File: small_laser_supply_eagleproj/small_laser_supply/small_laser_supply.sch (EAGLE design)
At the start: 25 parts, among them U1 LT6003_SOT23-5, X1 VIN, X2 CTRL, X3 OUT

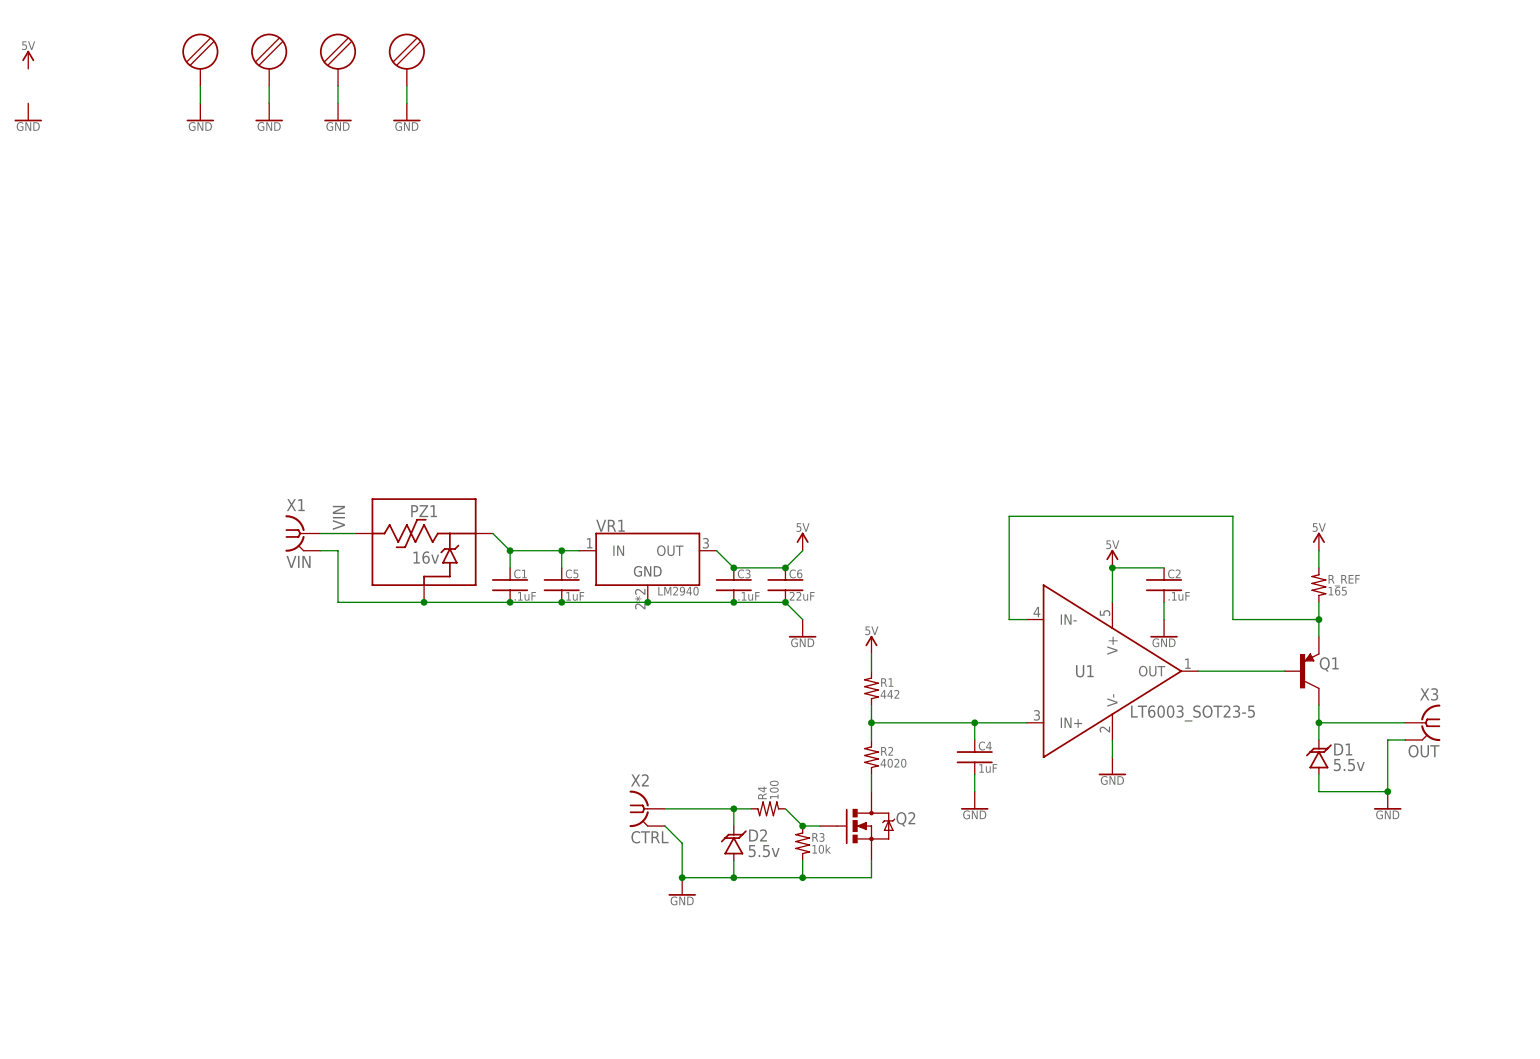
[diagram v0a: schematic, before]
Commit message: Fixed version of the schematic seems to be finished
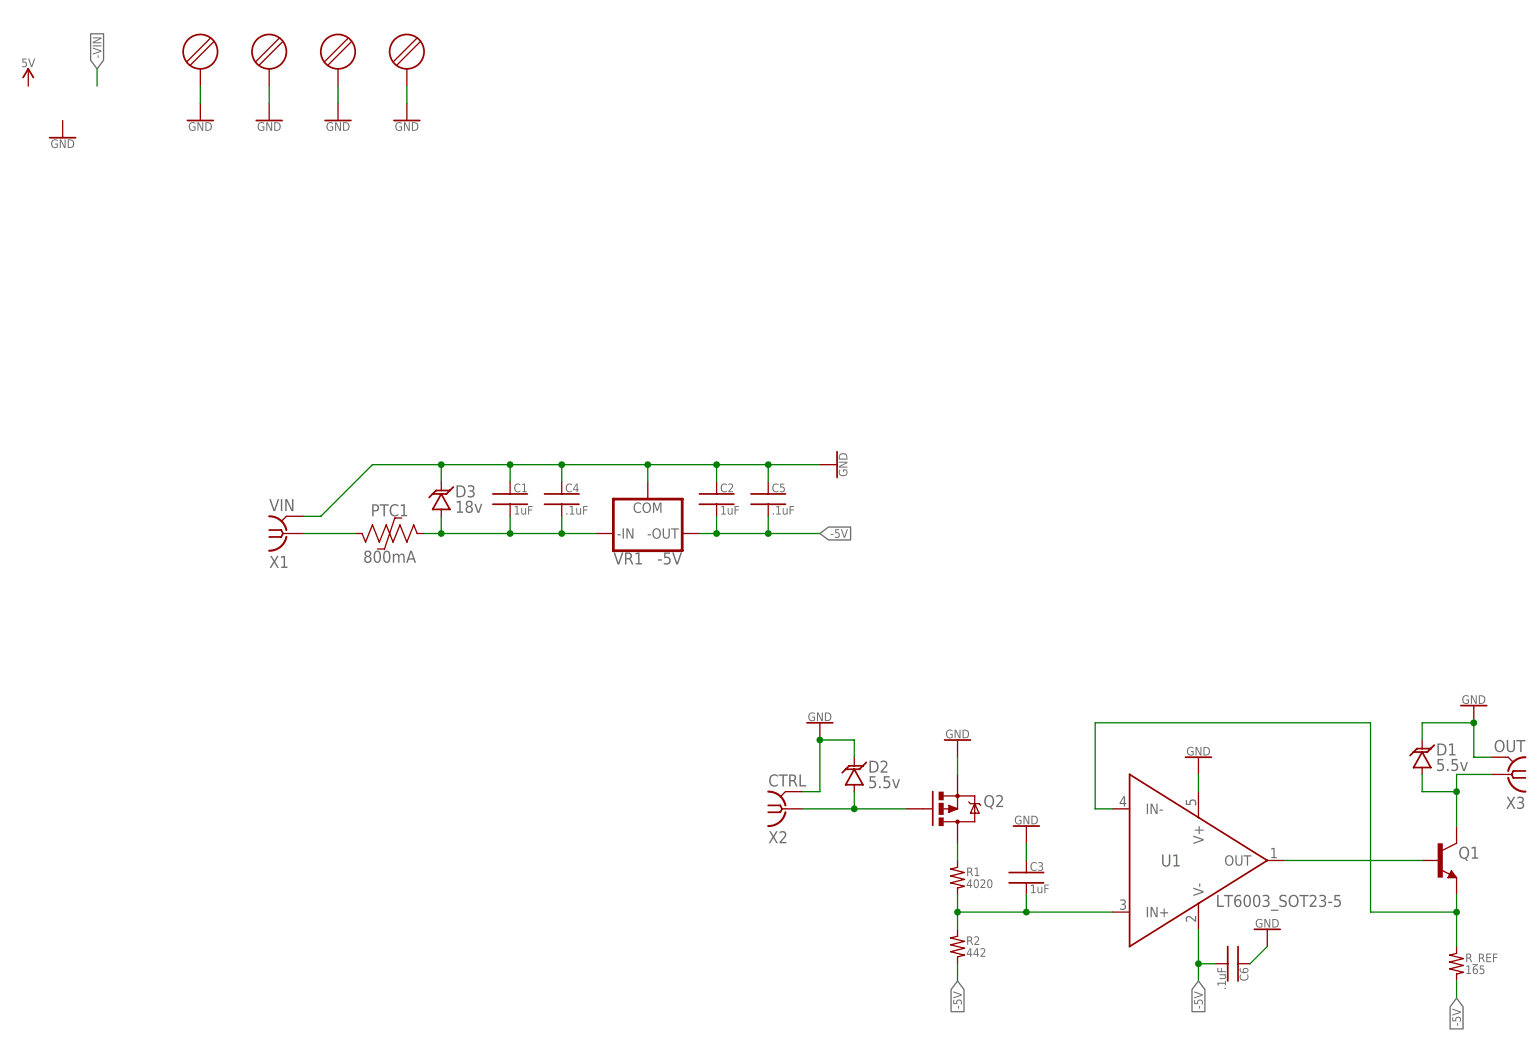
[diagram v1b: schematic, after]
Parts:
- removed PZ1: 16v, small_laser_supply_lib:POLYZEN_LS
- removed R3: 10k, small_laser_supply_lib:RES_0603
- removed R4: 100, small_laser_supply_lib:RES_0603
- added D3: 18v, small_laser_supply_lib:TVS-UNI_DO-214AA
- added PTC1: 800mA, small_laser_supply_lib:PTC_2SMD
- C1, C2, C3: value .1uF -> 1uF
- C4, C5: value 1uF -> .1uF
- C6: value 22uF -> .1uF; device small_laser_supply_lib:CAP_0805 -> small_laser_supply_lib:CAP_0603
- Q1: device small_laser_supply_lib:BJT_PNP_SOT23-3 -> small_laser_supply_lib:BJT_NPN_SOT23-3
- Q2: device small_laser_supply_lib:MOSFET_N-CHANNEL_SOT23-3 -> small_laser_supply_lib:MOSFET_P-CHANNEL_SOT23-3
- R1: value 442 -> 4020
- R2: value 4020 -> 442
- VR1: value (none) -> -5V; device small_laser_supply_lib:LM2940X_SOT-223 -> small_laser_supply_lib:79XX_VREG_DPAK
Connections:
- removed net 5V: C2.1, C3.1, C6.1, R1.1, R_REF.1, U1.V+, VR1.OUT
- removed net N$1 (its old number): Q1.E, R_REF.2, U1.IN-
- removed net N$5: Q2.D, R2.2
- removed net VIN: PZ1.V_IN, X1.1
- new net -5V: C2.2, C5.2, C6.2, R2.2, R_REF.2, U1.V-, VR1.OUT
- new net N$8: C1.2, C4.2, D3.A, PTC1.2, VR1.IN
- new net N$9: D2.A, Q2.G, X2.1
- net GND: now also C1.1, C2.1, C3.1, C4.1, C5.1, C6.1, D1.C, D2.C, D3.C, U1.V+; no longer C1.2, C2.2, C3.2, C4.2, C5.2, C6.2, D1.A, D2.A, PZ1.GND, R3.2, U1.V-
- net N$2: now also Q1.E, R_REF.1, U1.IN-; no longer D1.C, Q1.C, X3.1
- net N$3: now also Q2.D, R1.1; no longer C1.1, C5.1, PZ1.V_OUT, VR1.IN
- net N$4: now also PTC1.1, X1.1; no longer Q2.G, R3.1, R4.2
- net N$6: now also C3.2; no longer C4.1
- net N$7: now also D1.A, Q1.C, X3.1; no longer D2.C, R4.1, X2.1
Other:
- moved on the sheet: C1, C2, C3, C4, C5, C6, D1, D2, Q1, Q2, R1, R2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
